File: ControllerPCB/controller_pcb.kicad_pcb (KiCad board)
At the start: 2 copper layers, 16 parts, among them J1 USB3_A, U1 Pico, U2 AP63203WU

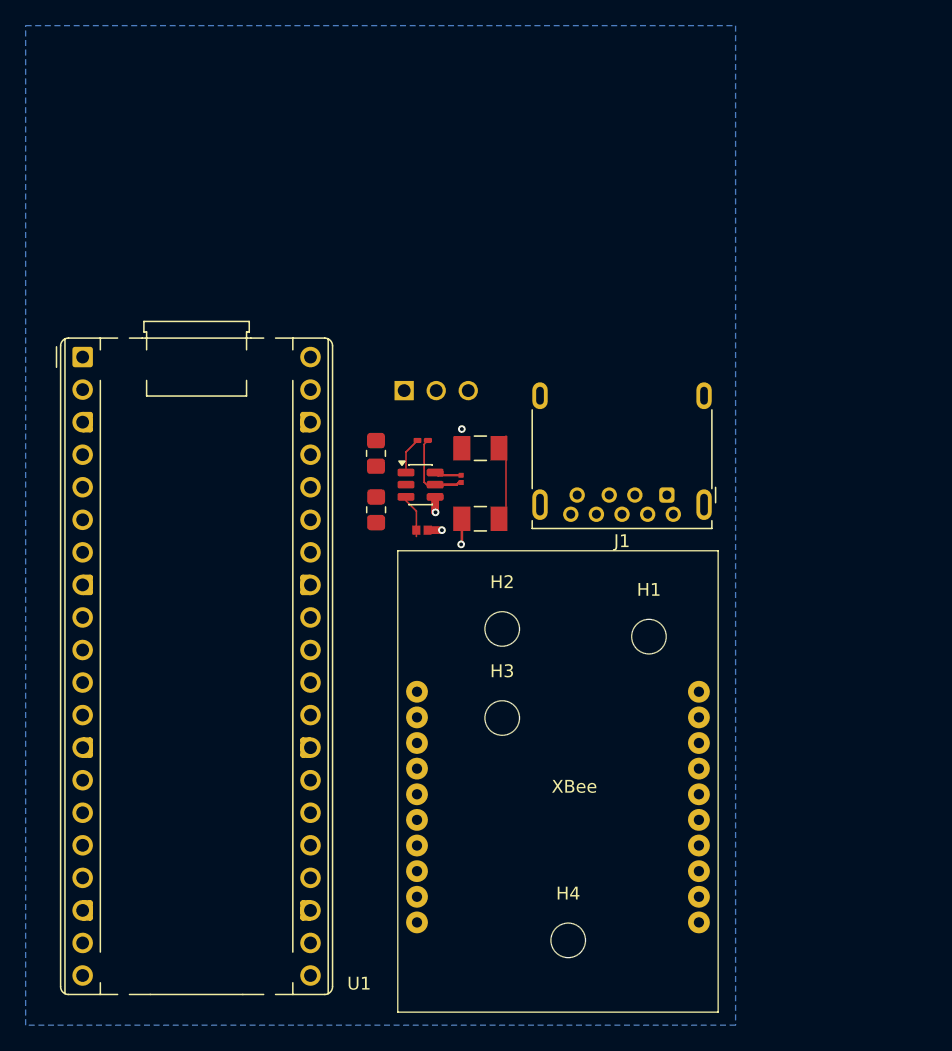
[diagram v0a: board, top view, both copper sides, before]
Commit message: controller pcb
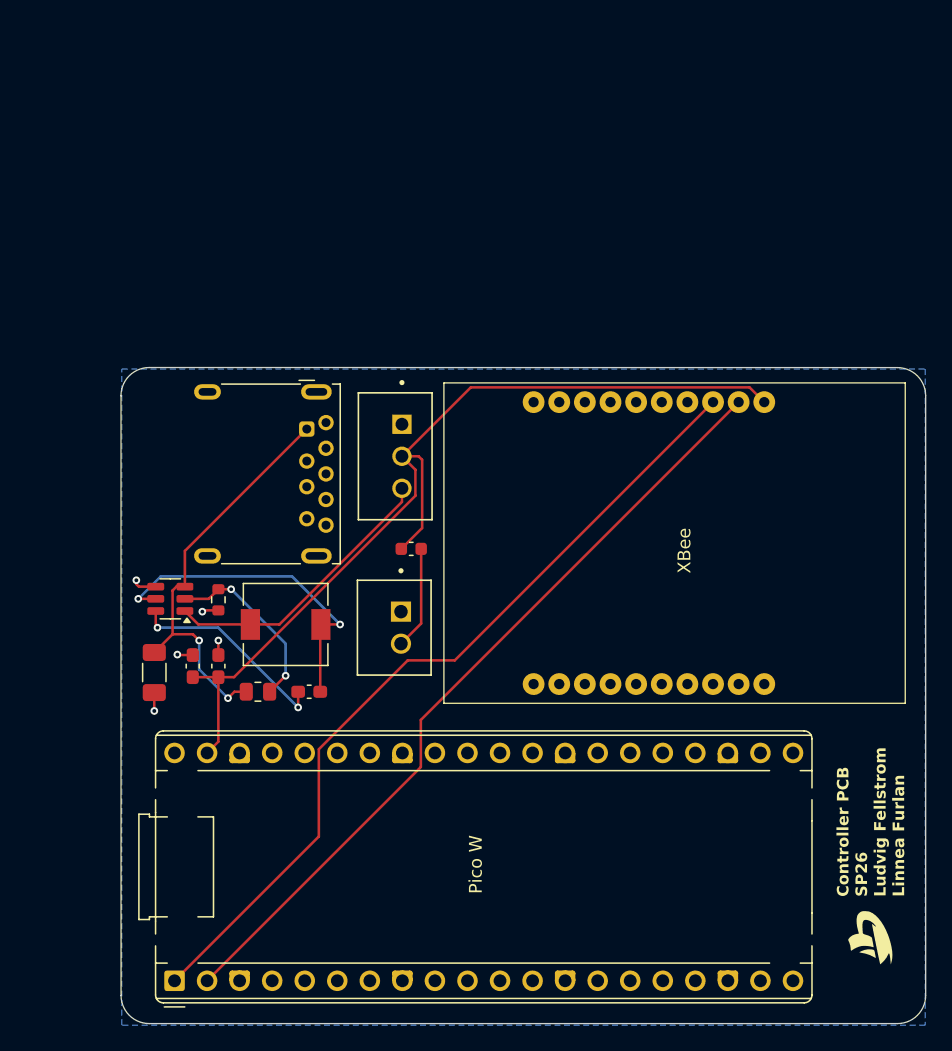
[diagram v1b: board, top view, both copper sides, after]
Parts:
- removed H1, H2, H3, H4: MountingHole, MountingHole:MountingHole_2.7mm
- removed R3a1, R3b1: 100k, Resistor_SMD:R_0805_2012Metric_Pad1.20x1.40mm_HandSolder
- removed the U2 at (112.8, 75.3)
- added D1: LED, switchbox_footprints:2_pin_header, F.Cu at (111.1, 87.0)
- added G***: LOGO, LOGO, F.Cu at (147.9, 110.6)
- added R1: 100, Capacitor_SMD:C_0603_1608Metric, F.Cu at (112.0, 80.3)
- added R3: 100k, Resistor_SMD:R_0805_2012Metric, F.Cu at (100.1, 91.5)
- added R_Buck_3: 100k, Resistor_SMD:R_0603_1608Metric, F.Cu at (97.0, 84.3)
- added U3: AP63203WU, Package_TO_SOT_SMD:TSOT-23-6, F.Cu at (93.2, 84.2)
- C1: footprint switchbox_footprints:CAPC1005X70N -> Capacitor_SMD:C_1206_3216Metric_Pad1.33x1.80mm_HandSolder
- C2: footprint switchbox_footprints:CAPC0603X33N -> Capacitor_SMD:C_0603_1608Metric_Pad1.08x0.95mm_HandSolder
- C3, C4: footprint switchbox_footprints:CAPC3216X190N -> Capacitor_SMD:C_0603_1608Metric_Pad1.08x0.95mm_HandSolder
- L1: footprint Inductor_SMD:L_0201_0603Metric_Pad0.64x0.40mm_HandSolder -> Inductor_SMD:L_6.3x6.3_H3
- PWR_SW1: moved to F.Cu
- moved U1 49.2 mm to (93.6, 114.1), turned to 90 degrees
- moved J1 28.6 mm to (103.9, 71.0), turned to -90 degrees
- moved C3 26.6 mm to (97.0, 89.5), turned to 90 degrees
- moved C4 25.2 mm to (95.0, 89.5), turned to 90 degrees
- moved C1 23.7 mm to (92.0, 90.0), turned to -90 degrees
- moved C2 20.4 mm to (104.1, 91.5), turned to 0 degrees
- moved U2 19.6 mm to (133.6, 80.4), turned to -90 degrees
- moved L1 17.9 mm to (102.2, 86.2)
- moved PWR_SW1 6.22 mm to (111.2, 73.3), turned to 90 degrees
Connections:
- C1 pad 1: Sys_Vin -> Net-(J1-VBUS)
- C3 pad 1: 3.3VBuck -> Net-(PWR_SW1-B)
- C4 pad 1: 3.3VBuck -> Net-(PWR_SW1-B)
- L1 pad 2: 3.3VBuck -> Net-(PWR_SW1-C)
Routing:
- net Net-(PWR_SW1-B): track 0.00 -> 73.3 mm
- net Net-(U1-GPIO0): track 0.00 -> 64.7 mm
- net /DOUT: track 0.00 -> 62.3 mm
- net Net-(J1-VBUS): track 0.00 -> 32.1 mm, vias 0 -> 2
- net Net-(PWR_SW1-C): track 0.00 -> 22.4 mm
- net Net-(U3-SW): track 6.41 -> 26.2 mm, vias 0 -> 2
- net Net-(U3-EN): track 0.00 -> 14.2 mm, vias 0 -> 2
- net Net-(U3-BST): track 2.12 -> 16.1 mm, vias 0 -> 2
- net 3.3VBuck: track 8.32 -> 0.00 mm
- net Net-(D1-A): track 0.00 -> 8.05 mm
- net Sys_Vin: track 3.42 -> 0.00 mm
- net GND: track 4.36 -> 6.98 mm, vias 4 -> 5
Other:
- board outline added: 62.8 x 51.2 mm
- board text added: "Controller PCB SP26 Ludvig Fellstrom Linnea Furlan"
- board text added: "Pico W"
